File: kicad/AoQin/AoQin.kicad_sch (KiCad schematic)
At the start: 12 parts, among them J1 1869253, J15 Conn_02x03_Odd_Even, J16 Conn_02x03_Odd_Even, J2 1869253, J3 1869253, J4 1869253, J5 1869253, J6 1869253, J7 Conn_02x03_Odd_Even, J8 Screw_Terminal_01x03, J9 Screw_Terminal_01x03

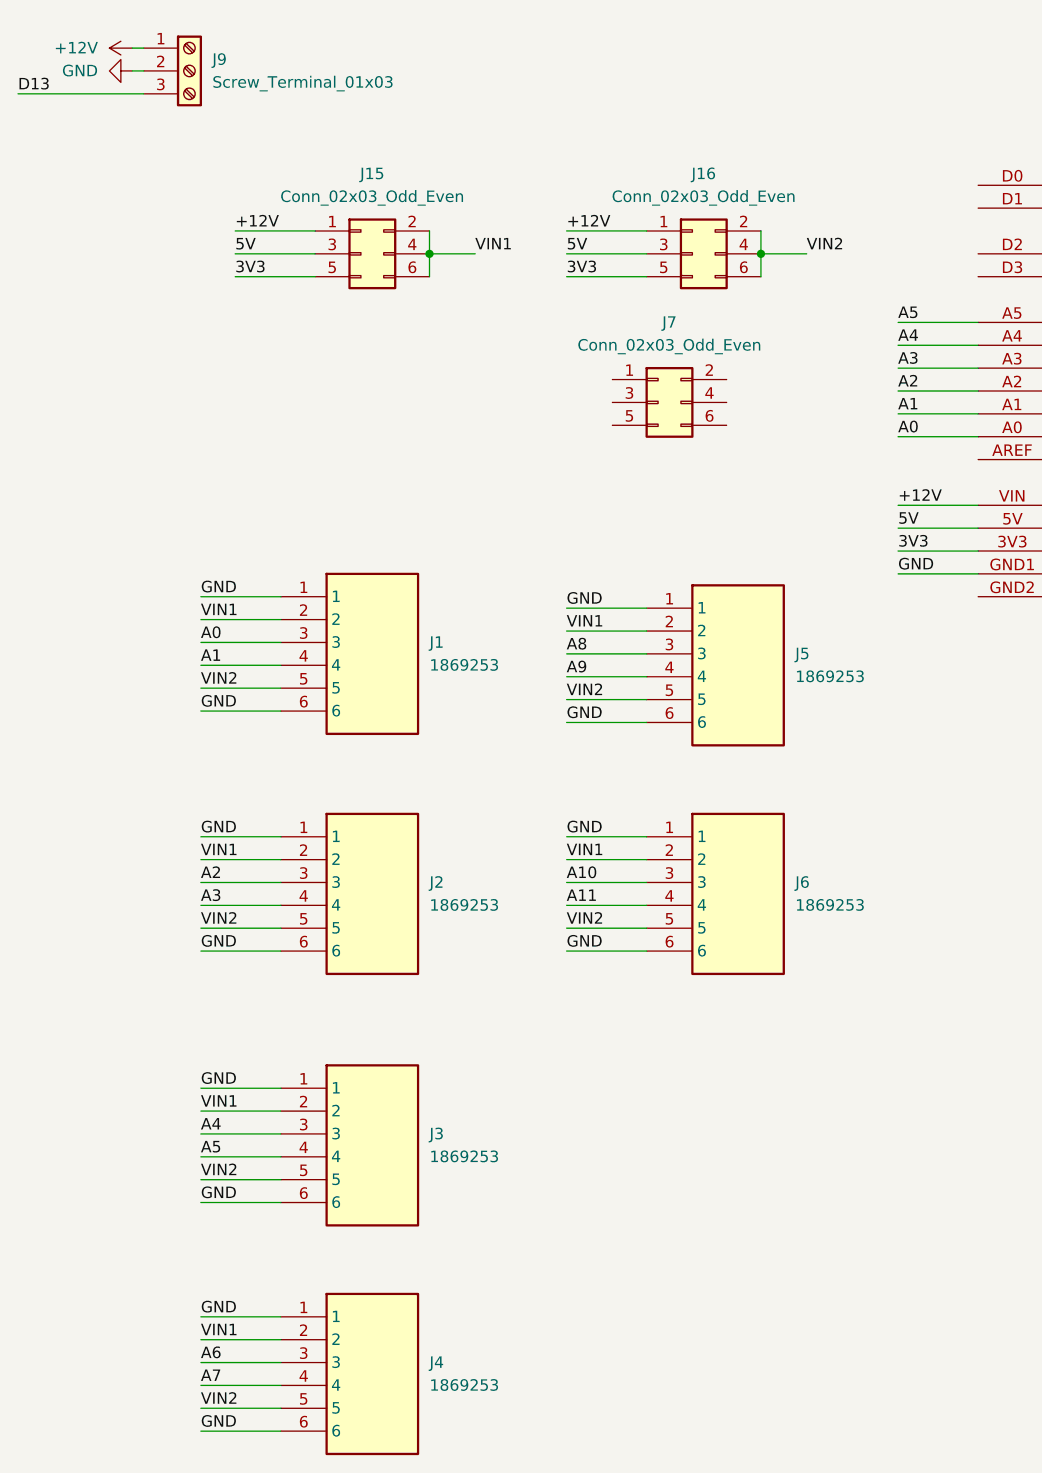
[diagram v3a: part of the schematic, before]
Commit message: Regrets… I've Had a Few
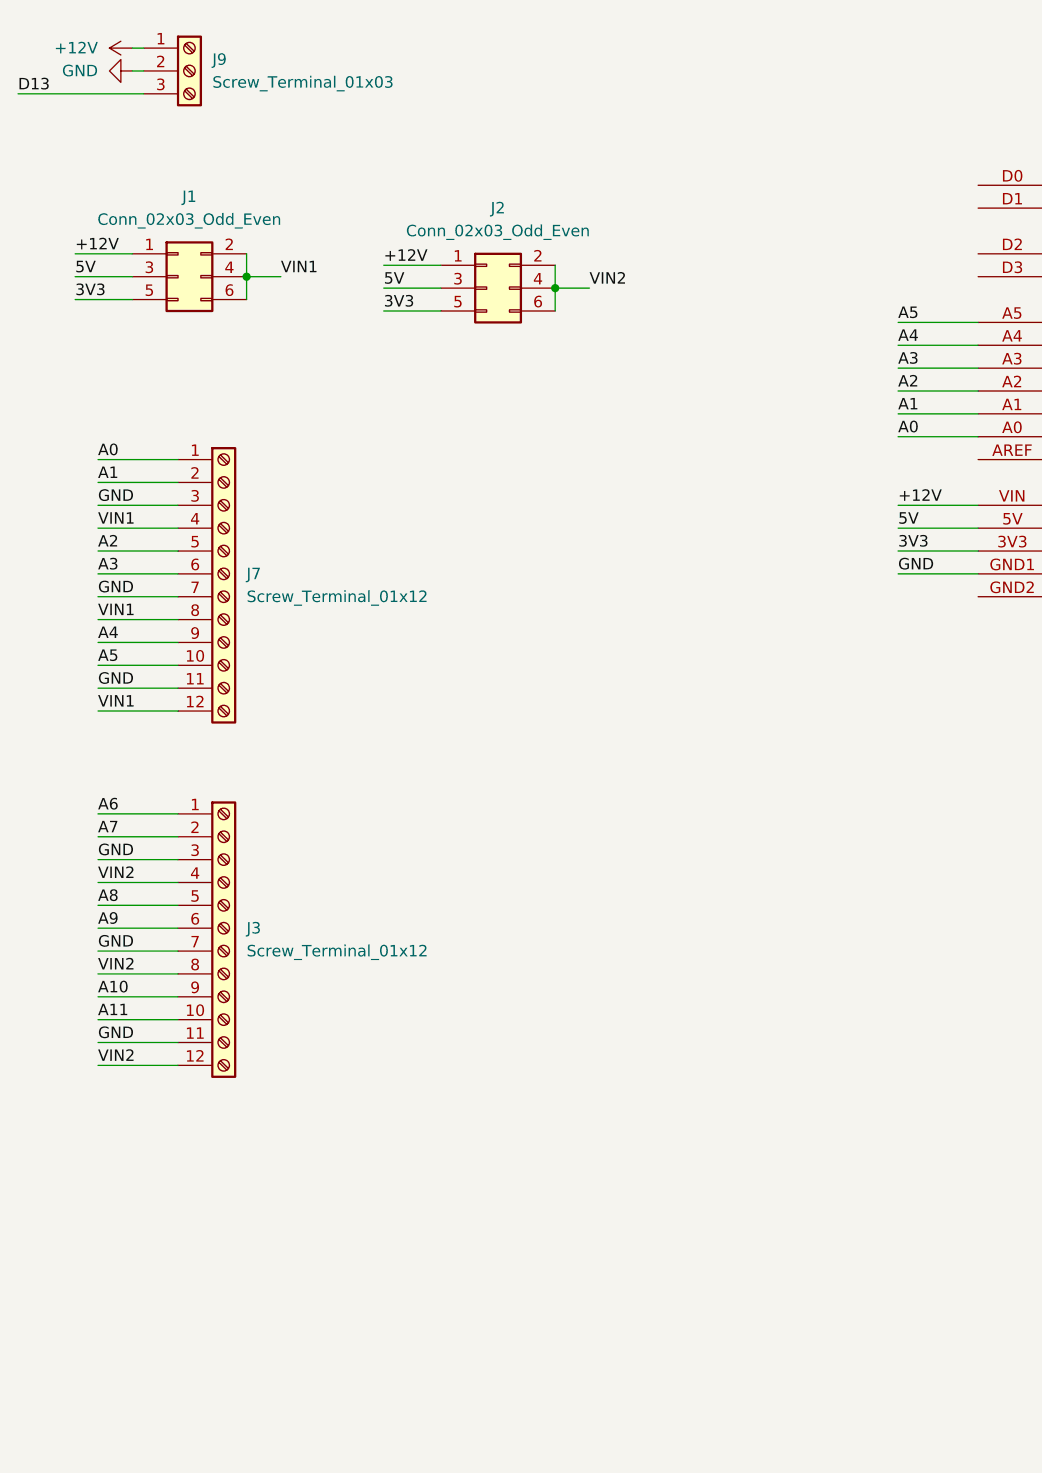
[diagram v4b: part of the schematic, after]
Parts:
- removed J1, J2, J3, J4, J5, J6: 1869253, footprints:SMKDSN_15_6_508, symbol PheonixContact:1869253
- removed J15, J16, J7: Conn_02x03_Odd_Even, Connector_PinHeader_2.54mm:PinHeader_2x03_P2.54mm_Vertical, symbol Connector_Generic:Conn_02x03_Odd_Even
- added J1, J2: Conn_02x03_Odd_Even, Connector_PinHeader_2.54mm:PinHeader_2x03_P2.54mm_Vertical, symbol Connector_Generic:Conn_02x03_Odd_Even
- added J3, J7: Screw_Terminal_01x12, footprints:1869318, symbol Connector:Screw_Terminal_01x12
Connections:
- net +12V: now also J1.1 (Pin_1), J2.1 (Pin_1)
- net 3V3: now also J1.5 (Pin_5), J2.5 (Pin_5)
- net 5V: now also J1.3 (Pin_3), J2.3 (Pin_3)
- net A0: now also J7.1 (Pin_1)
- net A1: now also J7.2 (Pin_2)
- net A10: now also J3.9 (Pin_9)
- net A11: now also J3.10 (Pin_10)
- net A2: now also J7.5 (Pin_5)
- net A3: now also J7.6 (Pin_6)
- net A4: now also J7.9 (Pin_9)
- net A5: now also J7.10 (Pin_10)
- net A6: now also J3.1 (Pin_1)
- net A7: now also J3.2 (Pin_2)
- net A8: now also J3.5 (Pin_5)
- net A9: now also J3.6 (Pin_6)
- net GND: now also J3.11 (Pin_11), J3.3 (Pin_3), J3.7 (Pin_7), J7.11 (Pin_11), J7.3 (Pin_3), J7.7 (Pin_7)
- net VIN1: now also J1.2 (Pin_2), J1.4 (Pin_4), J1.6 (Pin_6), J7.12 (Pin_12), J7.4 (Pin_4), J7.8 (Pin_8)
- net VIN2: now also J2.2 (Pin_2), J2.4 (Pin_4), J2.6 (Pin_6), J3.12 (Pin_12), J3.4 (Pin_4), J3.8 (Pin_8)

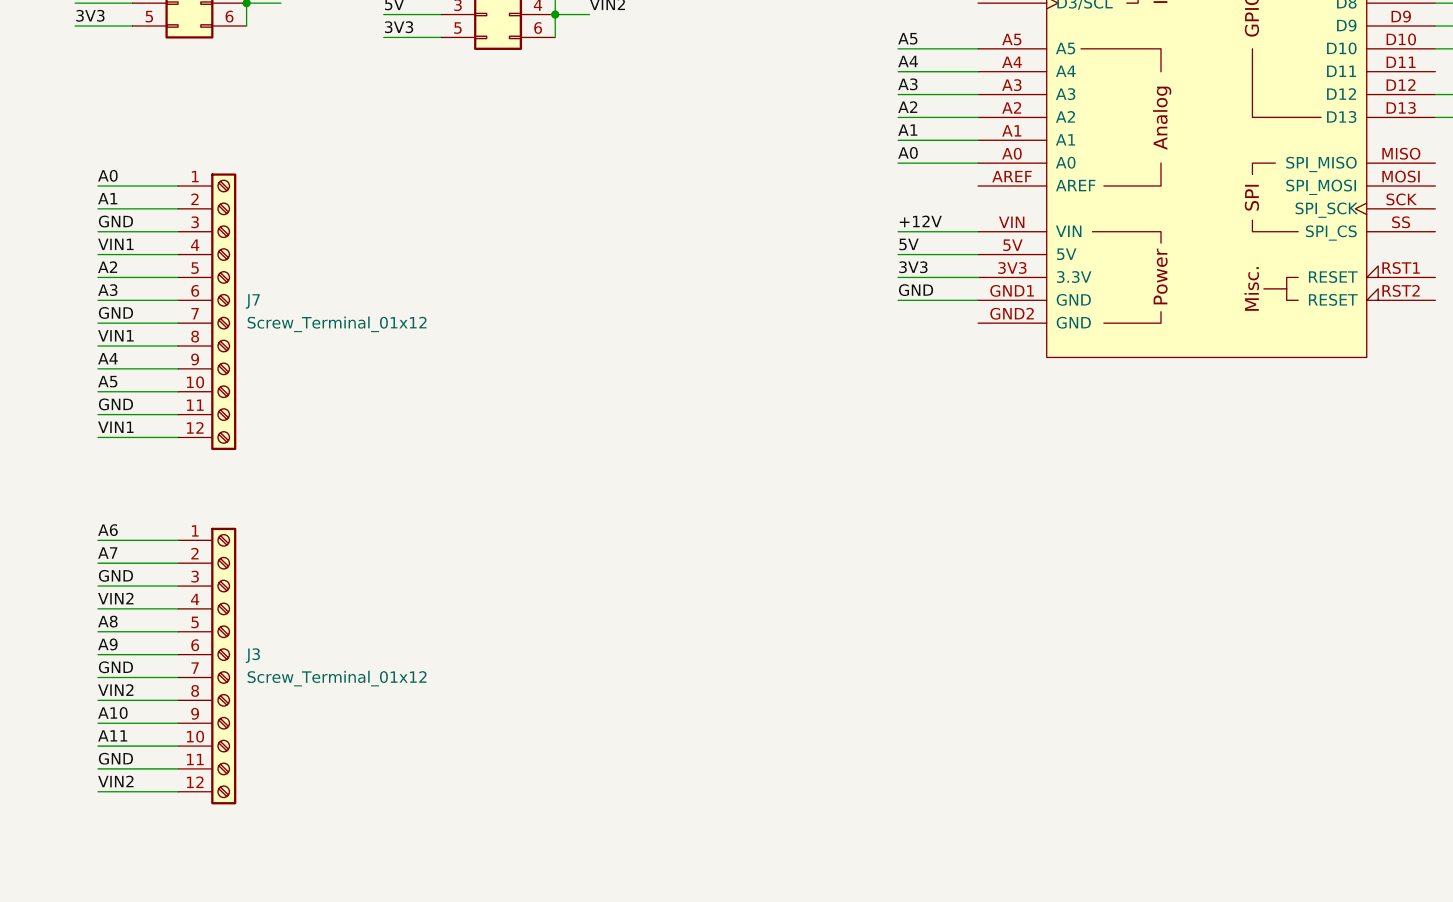
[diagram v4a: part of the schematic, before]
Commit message: Web of Desire
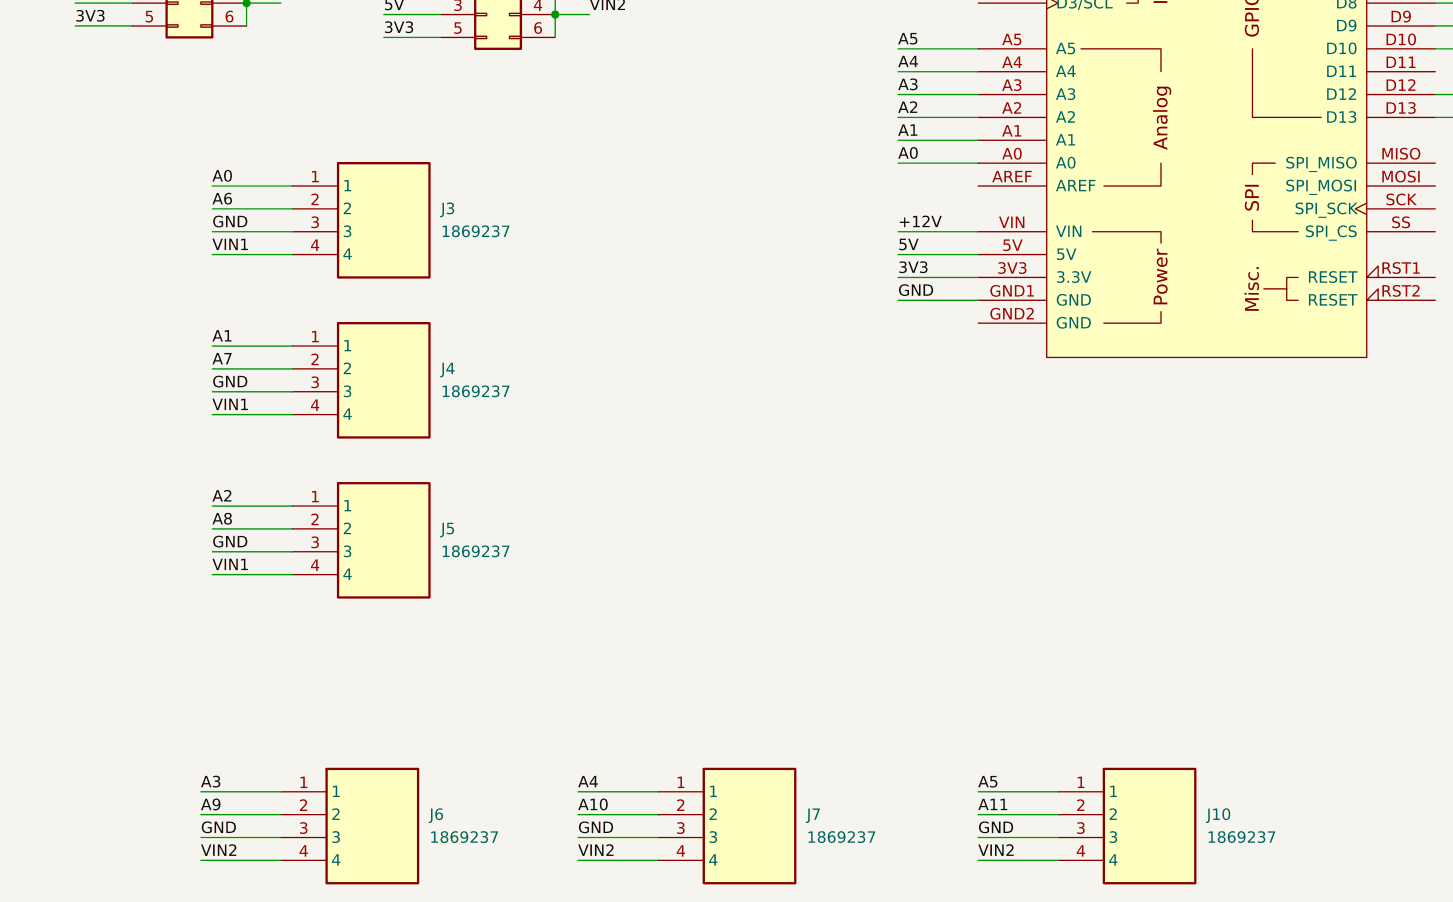
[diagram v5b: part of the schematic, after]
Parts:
- removed J3, J7: Screw_Terminal_01x12, footprints:1869318, symbol Connector:Screw_Terminal_01x12
- added J10, J3, J4, J5, J6, J7: 1869237, footprints:SMKDSN_15_4_508, symbol PheonixContact:1869237
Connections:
- net A0: now also J3.1
- net A1: now also J4.1
- net A10: now also J7.2
- net A11: now also J10.2
- net A2: now also J5.1
- net A3: now also J6.1
- net A4: now also J7.1
- net A5: now also J10.1
- net A6: now also J3.2
- net A7: now also J4.2
- net A8: now also J5.2
- net A9: now also J6.2
- net GND: now also J10.3, J3.3, J4.3, J5.3, J6.3, J7.3
- net VIN1: now also J3.4, J4.4, J5.4
- net VIN2: now also J10.4, J6.4, J7.4
